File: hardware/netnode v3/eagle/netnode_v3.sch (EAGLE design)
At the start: 26 parts, among them IC1 TSR-1, IC2 PIC18F4K80, IC3 FOD060L, X1 DC10R, X2 XPORT

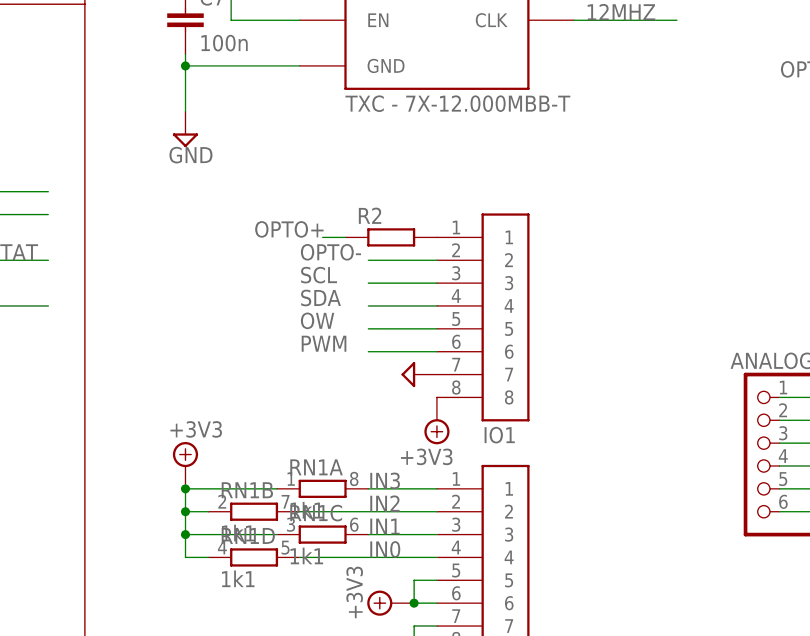
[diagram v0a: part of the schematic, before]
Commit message: Further finalization of board
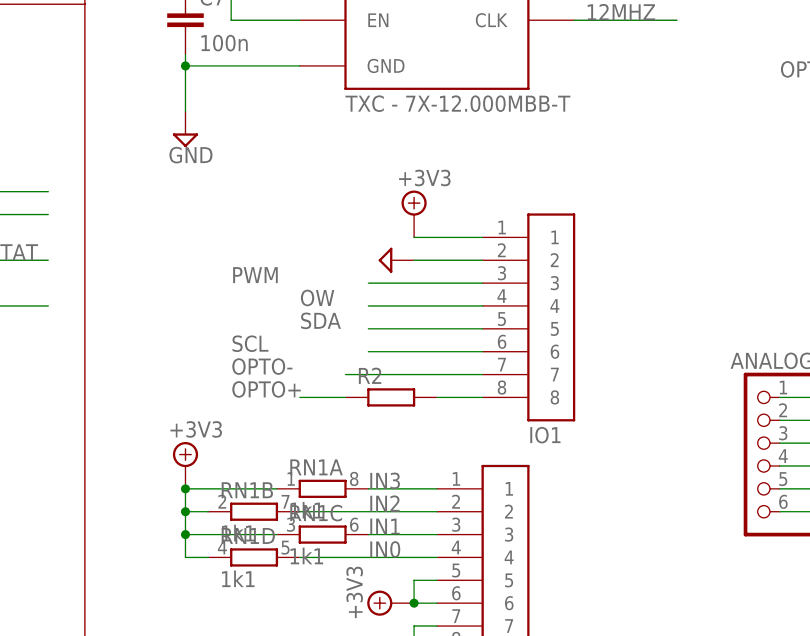
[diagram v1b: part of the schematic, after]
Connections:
- net +3V3: now also IO1.1; no longer IO1.8
- net GND: now also IO1.2; no longer IO1.7
- net N$3: now also IO1.8; no longer IO1.1
- net OPTO-: now also IO1.7; no longer IO1.2
- net OW: now also IO1.4; no longer IO1.5
- net PWM: now also IO1.3; no longer IO1.6
- net SCL: now also IO1.6; no longer IO1.3
- net SDA: now also IO1.5; no longer IO1.4
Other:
- moved on the sheet: IO1, R2
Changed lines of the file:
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@@
 </instance>
 <instance part="V5" gate="+3V3" x="10.16" y="63.5"/>
-<instance part="IO1" gate="G$1" x="139.7" y="48.26" smashed="yes">
-<attribute name="NAME" x="132.08" y="40.64" size="1.778" layer="95"/>
-<attribute name="OC_FARNELL" x="139.7" y="48.26" size="1.778" layer="96" rot="R90" display="off"/>
-<attribute name="MF" x="139.7" y="48.26" size="1.778" layer="96" rot="R90" display="off"/>
-<attribute name="MPN" x="139.7" y="48.26" size="1.778" layer="96" rot="R90" display="off"/>
+<instance part="IO1" gate="G$1" x="144.78" y="48.26" smashed="yes">
+<attribute name="NAME" x="137.16" y="40.64" size="1.778" layer="95"/>
+<attribute name="OC_FARNELL" x="144.78" y="48.26" size="1.778" layer="96" rot="R90" display="off"/>
+<attribute name="MF" x="144.78" y="48.26" size="1.778" layer="96" rot="R90" display="off"/>
+<attribute name="MPN" x="144.78" y="48.26" size="1.778" layer="96" rot="R90" display="off"/>
 </instance>
 <instance part="IO2" gate="G$1" x="139.7" y="20.32" smashed="yes">
@@
 <attribute name="MPN" x="203.2" y="93.98" size="1.778" layer="96" rot="R180" display="off"/>
 </instance>
-<instance part="V36" gate="GND" x="124.46" y="48.26" smashed="yes" rot="R270"/>
-<instance part="V37" gate="+3V3" x="127" y="43.18" rot="R180"/>
-<instance part="R2" gate="G$1" x="121.92" y="63.5"/>
+<instance part="V36" gate="GND" x="121.92" y="60.96" smashed="yes" rot="R270"/>
+<instance part="V37" gate="+3V3" x="124.46" y="66.04"/>
+<instance part="R2" gate="G$1" x="121.92" y="45.72"/>
 <instance part="RN3" gate="C" x="45.72" y="101.6" rot="R180"/>
 <instance part="RN3" gate="A" x="93.98" y="127" rot="R90"/>
@@
 </segment>
 <segment>
-<pinref part="IO1" gate="G$1" pin="7"/>
+<pinref part="IO1" gate="G$1" pin="2"/>
 <pinref part="V36" gate="GND" pin="GND"/>
+<wire x1="124.46" y1="60.96" x2="132.08" y2="60.96" width="0.1524" layer="91"/>
 </segment>
 </net>
@@
 </segment>
 <segment>
-<pinref part="IO1" gate="G$1" pin="8"/>
-<pinref part="V37" gate="+3V3" pin="+3V3"/>
-</segment>
-<segment>
 <pinref part="IC3" gate="G$1" pin="VCC"/>
 <wire x1="182.88" y1="101.6" x2="185.42" y2="101.6" width="0.1524" layer="91"/>
@@
 <pinref part="RN3" gate="C" pin="2"/>
 <wire x1="40.64" y1="101.6" x2="38.1" y2="101.6" width="0.1524" layer="91"/>
+</segment>
+<segment>
+<pinref part="IO1" gate="G$1" pin="1"/>
+<pinref part="V37" gate="+3V3" pin="+3V3"/>
+<wire x1="124.46" y1="63.5" x2="132.08" y2="63.5" width="0.1524" layer="91"/>
 </segment>
 </net>
@@
 <net name="SCL" class="1">
 <segment>
-<pinref part="IO1" gate="G$1" pin="3"/>
-<wire x1="127" y1="58.42" x2="119.38" y2="58.42" width="0.1524" layer="91"/>
-<label x="111.76" y="58.42" size="1.778" layer="95"/>
+<label x="104.14" y="50.8" size="1.778" layer="95"/>
+<pinref part="IO1" gate="G$1" pin="6"/>
+<wire x1="132.08" y1="50.8" x2="119.38" y2="50.8" width="0.1524" layer="91"/>
 </segment>
 <segment>
@@
 <net name="SDA" class="1">
 <segment>
-<pinref part="IO1" gate="G$1" pin="4"/>
-<wire x1="127" y1="55.88" x2="119.38" y2="55.88" width="0.1524" layer="91"/>
-<label x="111.76" y="55.88" size="1.778" layer="95"/>
-</segment>
-<segment>
 <pinref part="IC2" gate="G$1" pin="RC4/SDA/SDI"/>
 <wire x1="210.82" y1="160.02" x2="220.98" y2="160.02" width="0.1524" layer="91"/>
 <label x="213.36" y="160.02" size="1.778" layer="95"/>
 </segment>
+<segment>
+<pinref part="IO1" gate="G$1" pin="5"/>
+<wire x1="132.08" y1="53.34" x2="119.38" y2="53.34" width="0.1524" layer="91"/>
+<label x="111.76" y="53.34" size="1.778" layer="95"/>
+</segment>
 </net>
 <net name="OPTO+" class="1">
@@
 <segment>
 <pinref part="R2" gate="G$1" pin="1"/>
-<wire x1="116.84" y1="63.5" x2="114.3" y2="63.5" width="0.1524" layer="91"/>
-<label x="106.68" y="63.5" size="1.778" layer="95"/>
+<wire x1="116.84" y1="45.72" x2="111.76" y2="45.72" width="0.1524" layer="91"/>
+<label x="104.14" y="45.72" size="1.778" layer="95"/>
 </segment>
 </net>
@@
 </segment>
 <segment>
-<pinref part="IO1" gate="G$1" pin="2"/>
-<wire x1="127" y1="60.96" x2="119.38" y2="60.96" width="0.1524" layer="91"/>
-<label x="111.76" y="60.96" size="1.778" layer="95"/>
+<label x="104.14" y="48.26" size="1.778" layer="95"/>
+<pinref part="IO1" gate="G$1" pin="7"/>
+<wire x1="132.08" y1="48.26" x2="116.84" y2="48.26" width="0.1524" layer="91"/>
 </segment>
 </net>
@@
 </segment>
 <segment>
-<pinref part="IO1" gate="G$1" pin="5"/>
-<wire x1="127" y1="53.34" x2="119.38" y2="53.34" width="0.1524" layer="91"/>
-<label x="111.76" y="53.34" size="1.778" layer="95"/>
+<pinref part="IO1" gate="G$1" pin="4"/>
+<wire x1="132.08" y1="55.88" x2="119.38" y2="55.88" width="0.1524" layer="91"/>
+<label x="111.76" y="55.88" size="1.778" layer="95"/>
 </segment>
 </net>
@@
 </segment>
 <segment>
-<pinref part="IO1" gate="G$1" pin="6"/>
-<wire x1="127" y1="50.8" x2="119.38" y2="50.8" width="0.1524" layer="91"/>
-<label x="111.76" y="50.8" size="1.778" layer="95"/>
+<pinref part="IO1" gate="G$1" pin="3"/>
+<wire x1="132.08" y1="58.42" x2="119.38" y2="58.42" width="0.1524" layer="91"/>
+<label x="104.14" y="58.42" size="1.778" layer="95"/>
 </segment>
 </net>
@@
 </segment>
 </net>
-<net name="N$3" class="0">
-<segment>
-<pinref part="IO1" gate="G$1" pin="1"/>
-<pinref part="R2" gate="G$1" pin="2"/>
-</segment>
-</net>
 <net name="N$2" class="0">
 <segment>
@@
 </segment>
 </net>
+<net name="N$3" class="0">
+<segment>
+<pinref part="IO1" gate="G$1" pin="8"/>
+<pinref part="R2" gate="G$1" pin="2"/>
+<wire x1="127" y1="45.72" x2="132.08" y2="45.72" width="0.1524" layer="91"/>
+</segment>
+</net>
